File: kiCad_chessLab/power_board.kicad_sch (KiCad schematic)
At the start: 4 parts, among them IC66 TP4056, J4 DATA, J5 PWR

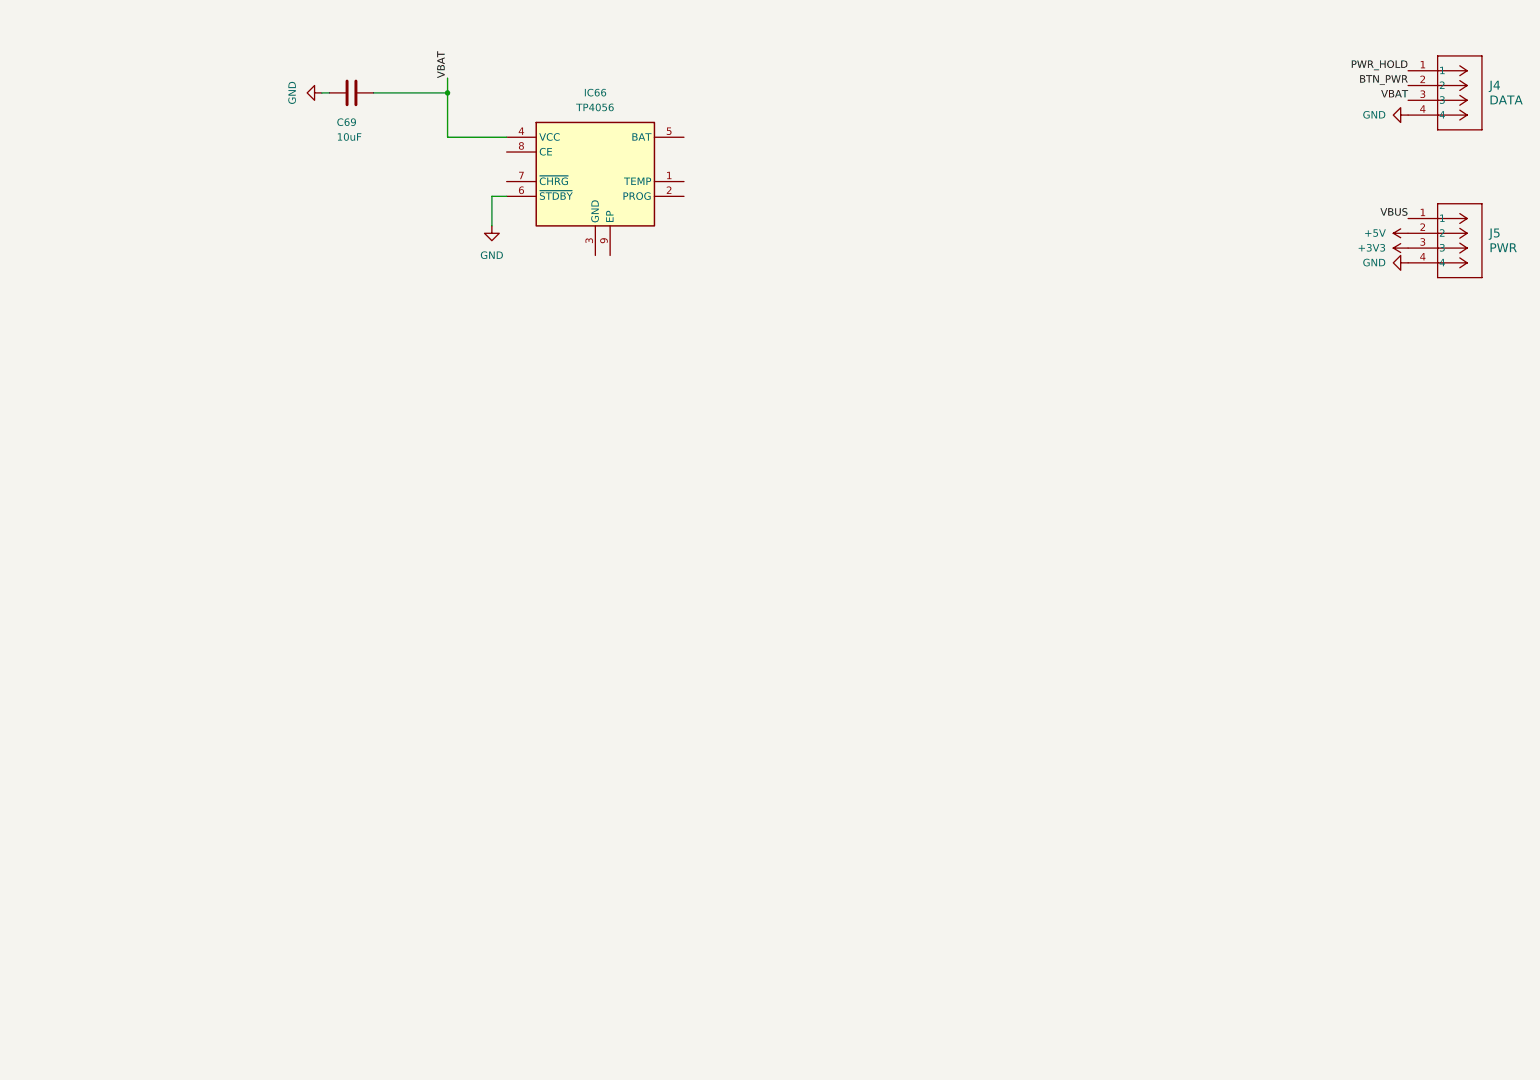
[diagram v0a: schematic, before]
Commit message: Complete Schematics
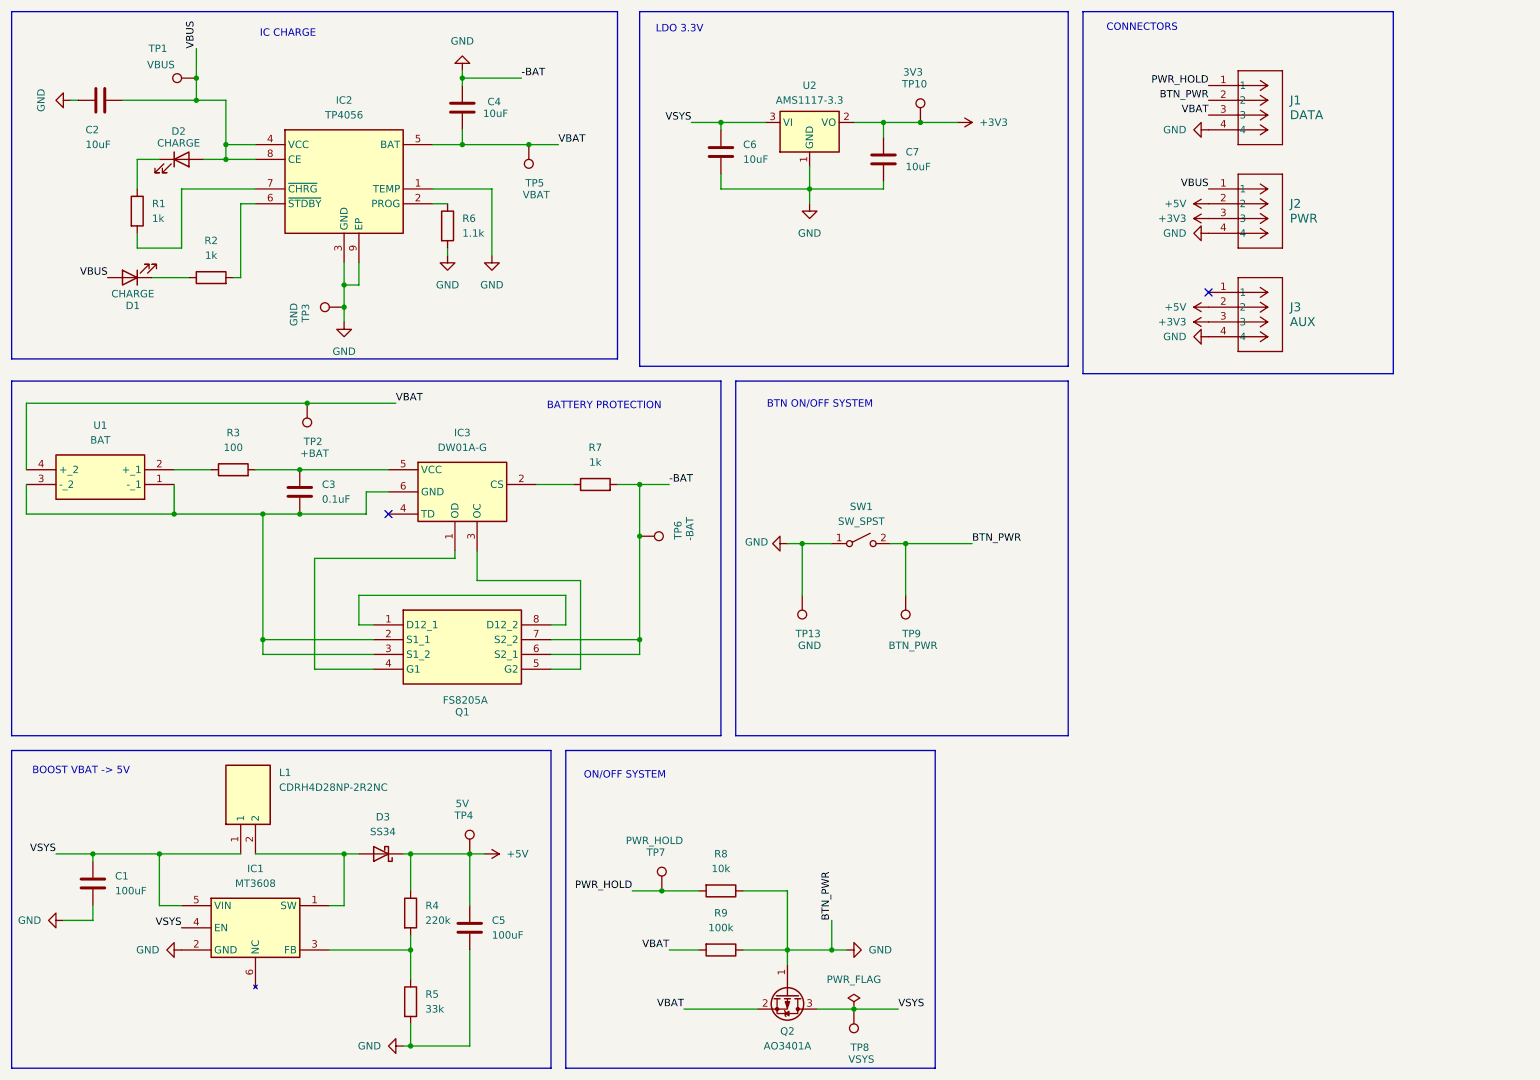
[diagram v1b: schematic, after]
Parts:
- added C1, C5: 100uF, Capacitor_SMD:C_1206_3216Metric_Pad1.33x1.80mm_HandSolder, symbol Device:C
- added C3: 0.1uF, Capacitor_SMD:C_0603_1608Metric_Pad1.08x0.95mm_HandSolder, symbol Device:C
- added C4, C6, C7: 10uF, Capacitor_SMD:C_0603_1608Metric_Pad1.08x0.95mm_HandSolder, symbol Device:C
- added D1, D2: CHARGE, LED_SMD:LED_0603_1608Metric_Pad1.05x0.95mm_HandSolder, symbol Device:LED
- added D3: SS34, Diode_SMD:D_SMA, symbol Diode:SS34
- added IC1: MT3608, SOT95P280X145-6N, symbol chessLab-symbols:MT3608
- added IC3: DW01A-G, chessLab-footprints:SOT95P280X135-6N, symbol chessLab-symbols:DW01A-G
- added J3: AUX, CONN4_1048_KEY, symbol chessLab-symbols:1048
- added L1: CDRH4D28NP-2R2NC, chessLab-footprints:CDRH4D28NP100NC, symbol chessLab-symbols:CDRH4D28NP-2R2NC
- added Q1: FS8205A, chessLab-footprints:SOP65P640X120-8N, symbol chessLab-symbols:FS8205A
- added Q2: AO3401A, Package_TO_SOT_SMD:SOT-23_Handsoldering, symbol Transistor_FET:AO3401A
- added R1, R2, R7: 1k, Resistor_SMD:R_0603_1608Metric_Pad0.98x0.95mm_HandSolder, symbol Device:R
- added R3: 100, Resistor_SMD:R_0603_1608Metric_Pad0.98x0.95mm_HandSolder, symbol Device:R
- added R4: 220k, Resistor_SMD:R_0603_1608Metric_Pad0.98x0.95mm_HandSolder, symbol Device:R
- added R5: 33k, Resistor_SMD:R_0603_1608Metric_Pad0.98x0.95mm_HandSolder, symbol Device:R
- added R6: 1.1k, Resistor_SMD:R_0603_1608Metric_Pad0.98x0.95mm_HandSolder, symbol Device:R
- added R8: 10k, Resistor_SMD:R_0603_1608Metric_Pad0.98x0.95mm_HandSolder, symbol Device:R
- added R9: 100k, Resistor_SMD:R_0603_1608Metric_Pad0.98x0.95mm_HandSolder, symbol Device:R
- added SW1: SW_SPST, symbol Switch:SW_SPST
- added TP1: VBUS, TestPoint:TestPoint_Plated_Hole_D2.0mm, symbol Connector:TestPoint
- added TP10: 3V3, TestPoint:TestPoint_Plated_Hole_D2.0mm, symbol Connector:TestPoint
- added TP13, TP3: GND, TestPoint:TestPoint_Plated_Hole_D2.0mm, symbol Connector:TestPoint
- added TP2: +BAT, TestPoint:TestPoint_Plated_Hole_D2.0mm, symbol Connector:TestPoint
- added TP4: 5V, TestPoint:TestPoint_Plated_Hole_D2.0mm, symbol Connector:TestPoint
- added TP5: VBAT, TestPoint:TestPoint_Plated_Hole_D2.0mm, symbol Connector:TestPoint
- added TP6: -BAT, TestPoint:TestPoint_Plated_Hole_D2.0mm, symbol Connector:TestPoint
- added TP7: PWR_HOLD, TestPoint:TestPoint_Plated_Hole_D2.0mm, symbol Connector:TestPoint
- added TP8: VSYS, TestPoint:TestPoint_Plated_Hole_D2.0mm, symbol Connector:TestPoint
- added TP9: BTN_PWR, TestPoint:TestPoint_Plated_Hole_D2.0mm, symbol Connector:TestPoint
- added U1: BAT, chessLab-footprints:x218650smd, symbol chessLab-symbols:1048
- added U2: AMS1117-3.3, Package_TO_SOT_SMD:SOT-223-3_TabPin2, symbol Regulator_Linear:AMS1117-3.3
- renumbered C69 to C2, IC66 to IC2, J4 to J1, J5 to J2
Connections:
- net BTN_PWR is gone; now on net GND: J1.2
- net +3V3: now also C7.1, J3.3, TP10.1, U2.2 (VO)
- net +5V: now also C5.1, D3.1 (K), J3.2, R4.1, TP4.1
- net GND: now also IC2.1 (TEMP), IC2.3 (GND), IC2.9 (EP), C1.2, C4.2, C5.2, C6.2, C7.2, IC1.2 (GND), J3.4, Q1.6 (S2_1), Q1.7 (S2_2), Q2.1 (G), R5.2, R6.2, R7.2, R8.1, R9.1, SW1.1 (A), SW1.2 (B), TP13.1, TP3.1, TP6.1, TP9.1, U2.1 (GND); no longer IC2.6 (~{STDBY})
- net PWR_HOLD: now also R8.2, TP7.1
- net VBAT: now also IC2.5 (BAT), C4.1, Q2.2 (S), R9.2, TP2.1, TP5.1, U1.4 (+_2); no longer C2.2, IC2.4 (VCC)
- net VBUS: now also C2.2, IC2.4 (VCC), IC2.8 (CE), D1.2 (A), D2.2 (A), TP1.1
- net at IC2.2 (PROG): now also R6.1
- net at IC2.7 (~{CHRG}): now also R1.2
- new net: D1.1 (K), R2.1
- new net: IC2.6 (~{STDBY}), R2.2
- new net: IC1.3 (FB), R4.2, R5.1
- new net: C3.2, IC3.6 (GND), Q1.2 (S1_1), Q1.3 (S1_2), U1.1 (-_1), U1.3 (-_2)
- new net: R3.1, U1.2 (+_1)
- new net: IC3.1 (OD), Q1.4 (G1)
- new net: IC3.2 (CS), R7.1
- new net: IC3.3 (OC), Q1.5 (G2)
- new net: C3.1, IC3.5 (VCC), R3.2
- new net: D2.1 (K), R1.1
- new net: Q1.1 (D12_1), Q1.8 (D12_2)
- new net: D3.2 (A), IC1.1 (SW), L1.2
- new net VSYS: C1.1, C6.1, IC1.4 (EN), IC1.5 (VIN), L1.1, Q2.3 (D), TP8.1, U2.3 (VI)
- no-connect marks 0 -> 2
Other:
- note added: "BATTERY PROTECTION"
- note added: "BOOST VBAT -> 5V"
- note added: "BTN ON/OFF SYSTEM"
- note added: "CONNECTORS"
- note added: "IC CHARGE"
- note added: "LDO 3.3V"
- note added: "ON/OFF SYSTEM"
- moved on the sheet: C2, IC2, J1, J2
